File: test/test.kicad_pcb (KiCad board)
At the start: 2 copper layers, 100 x 100 mm, 107 parts, among them J1 UEXT_Host, J2 Conn_01x02, J3 Conn_02x06_Odd_Even, J4 Conn_02x06_Odd_Even, J5 Conn_02x06_Odd_Even, Q1 BC859, Q10 BC848, Q11 BC808, Q12 BC848, Q13 BC848, Q14 BC808, Q15 BC848, Q16 BC808, Q17 BC808, Q2 BC859, Q3 BC859, Q4 BC859, Q5 BC859, Q6 BC848, Q7 BC808, Q8 BC848, Q9 BC808, U3 PCA9531PW, U4 PCF8574AT, U6 TLC59108FPW

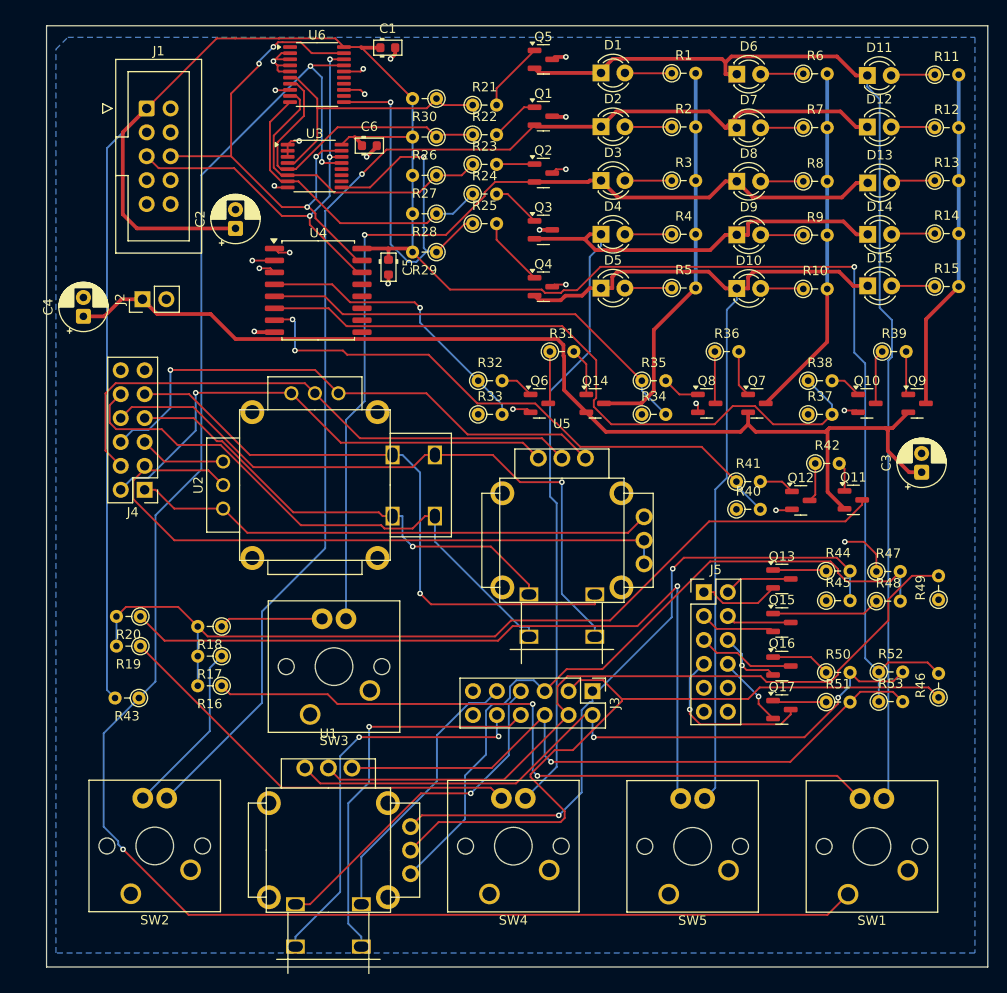
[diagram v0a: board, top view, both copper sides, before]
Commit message: work on 2nd update test
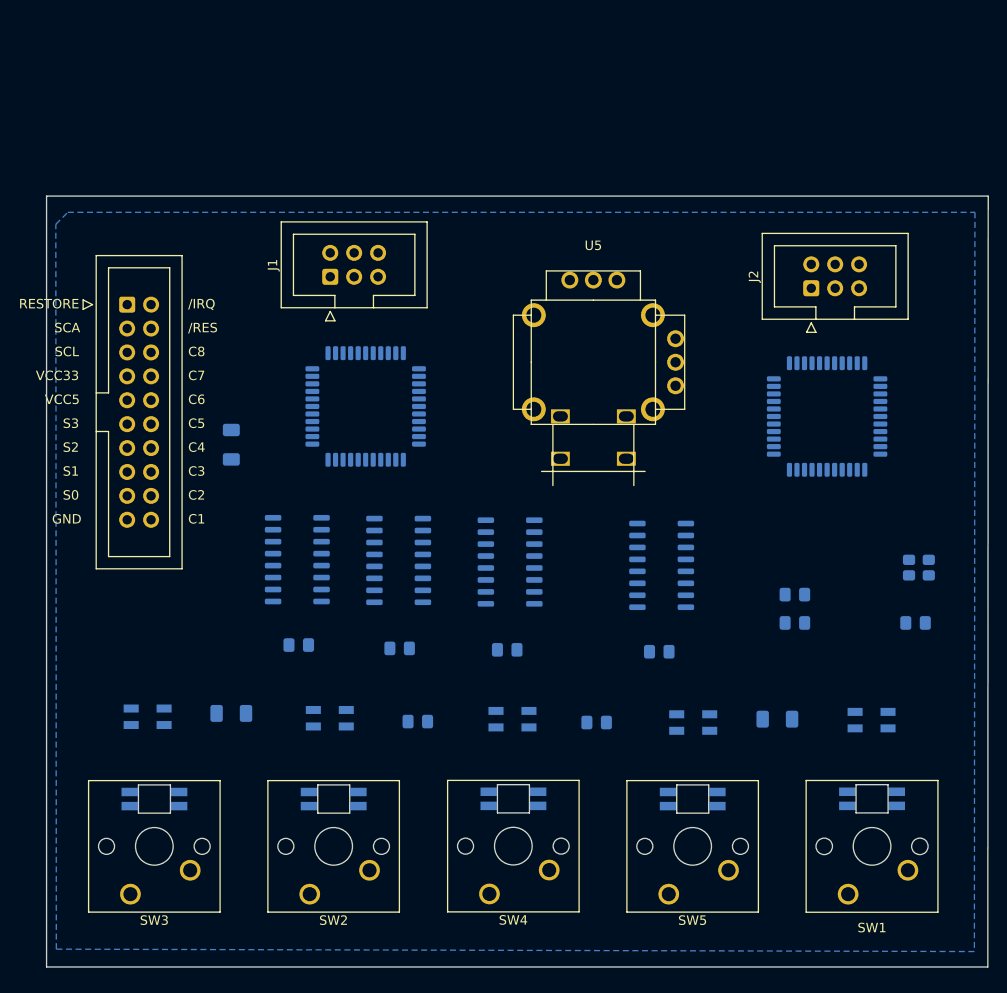
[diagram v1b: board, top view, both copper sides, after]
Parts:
- removed C1, C5, C6: C, PCM_Diode_SMD_Handsoldering_AKL:D_0603_1608Metric
- removed C2, C3, C4: C_Polarized, Capacitor_THT:CP_Radial_D5.0mm_P2.00mm
- removed D10, D11, D12, D13, D14, D15, D6, D7, D8, D9: LED, LED_THT:LED_D3.0mm
- removed J3, J4, J5: Conn_02x06_Odd_Even, Connector_PinHeader_2.54mm:PinHeader_2x06_P2.54mm_Vertical
- removed Q1, Q2, Q3, Q4, Q5: BC859, Package_TO_SOT_SMD:SOT-23
- removed Q10, Q12, Q13, Q15, Q6, Q8: BC848, Package_TO_SOT_SMD:SOT-23
- removed Q11, Q14, Q16, Q17, Q7, Q9: BC808, Package_TO_SOT_SMD:SOT-23
- removed R1, R10, R11, R12, R13, R14, R15, R16, R17, R18, R19, R2, R20, R3, R4, R5, R6, R7, R8, R9: R, Resistor_THT:R_Axial_DIN0204_L3.6mm_D1.6mm_P2.54mm_Vertical
- removed R21, R22, R23, R24, R25, R26, R27, R28, R29, R30, R31, R32, R33, R34, R35, R36, R37, R38, R39, R40, R41, R42, R43, R44, R45, R47, R48, R50, R51, R52, R53: 100k, Resistor_THT:R_Axial_DIN0204_L3.6mm_D1.6mm_P2.54mm_Vertical
- removed R46, R49: 1k, Resistor_THT:R_Axial_DIN0204_L3.6mm_D1.6mm_P2.54mm_Vertical
- removed U1: ~, petkn:THB Miniature Thumbstick THB001P
- added C10: 100n, Capacitor_SMD:C_0805_2012Metric_Pad1.18x1.45mm_HandSolder, B.Cu at (62.9, 127.3)
- added C11: 100n, Capacitor_SMD:C_0805_2012Metric_Pad1.18x1.45mm_HandSolder, B.Cu at (51.5, 127.2)
- added C12: 100n, Capacitor_SMD:C_0805_2012Metric_Pad1.18x1.45mm_HandSolder, B.Cu at (40.8, 126.8)
- added C13: 100n, Capacitor_SMD:C_0805_2012Metric_Pad1.18x1.45mm_HandSolder, B.Cu at (106.3, 124.4)
- added C14: 100n, Capacitor_SMD:C_0805_2012Metric_Pad1.18x1.45mm_HandSolder, B.Cu at (72.4, 135.0)
- added C15: 100u, Capacitor_SMD:C_1206_3216Metric_Pad1.33x1.80mm_HandSolder, B.Cu at (91.6, 134.7)
- added C16: 100u, Capacitor_SMD:C_1206_3216Metric_Pad1.33x1.80mm_HandSolder, B.Cu at (33.6, 134.1)
- added C17: 100n, Capacitor_SMD:C_0805_2012Metric_Pad1.18x1.45mm_HandSolder, B.Cu at (53.4, 134.9)
- added C18: 100u, Capacitor_SMD:C_1206_3216Metric_Pad1.33x1.80mm_HandSolder, B.Cu at (33.6, 105.5)
- added C7: 100n, Capacitor_SMD:C_0805_2012Metric_Pad1.18x1.45mm_HandSolder, B.Cu at (93.5, 124.4)
- added C8: 100n, Capacitor_SMD:C_0805_2012Metric_Pad1.18x1.45mm_HandSolder, B.Cu at (93.5, 121.4)
- added C9: 100n, Capacitor_SMD:C_0805_2012Metric_Pad1.18x1.45mm_HandSolder, B.Cu at (79.1, 127.5)
- added J6: New_PET_keyboard_connector, petkn:PET_New_Keyboard_Connector, F.Cu at (25.1, 100.8)
- added U7: 74LS145, Package_SO:SO-16_3.9x9.9mm_P1.27mm, B.Cu at (79.3, 118.3)
- added U8: ATmega32A-A, Package_QFP:TQFP-44_10x10mm_P0.8mm, B.Cu at (96.9, 102.5)
- added Y1: ASE-xxxMHz, Oscillator:Oscillator_SMD_Abracon_ASE-4Pin_3.2x2.5mm, B.Cu at (106.7, 118.6)
- D1, D2, D3, D4, D5: value LED -> SK6812MINI; footprint LED_THT:LED_D3.0mm -> LED_SMD:LED_SK6812MINI_PLCC4_3.5x3.5mm_P1.75mm; moved to B.Cu
- J1: value UEXT_Host -> AVR-ISP-6; footprint Connector_IDC:IDC-Header_2x05_P2.54mm_Vertical -> Connector_IDC:IDC-Header_2x03_P2.54mm_Vertical
- J2: value Conn_01x02 -> AVR-ISP-6; footprint Connector_PinHeader_2.54mm:PinHeader_1x02_P2.54mm_Vertical -> Connector_IDC:IDC-Header_2x03_P2.54mm_Vertical
- SW1: footprint petkn:SW_Cherry_MX_1.00u_PCB_with_LED -> CherryMX_PCB_LTST-A683CEGBW-Rotated:CherryMX_1.00u_PCB_LTST-A683CEGBW-Rotated
- SW2: value ~ -> CherryMX_LTST-A683CEGBW; footprint petkn:SW_Cherry_MX_1.00u_PCB_with_LED -> petkn:SW_Cherry_MX_1.00u_PCB_with_RGB_LED
- SW3, SW4, SW5: footprint petkn:SW_Cherry_MX_1.00u_PCB_with_LED -> petkn:SW_Cherry_MX_1.00u_PCB_with_RGB_LED
- U2: value ~ -> ATmega32A-A; footprint petkn:true-components-98002c3-ps2-ps3 -> Package_QFP:TQFP-44_10x10mm_P0.8mm; moved to B.Cu
- U3: value PCA9531PW -> 74HCT85; footprint Package_SO:TSSOP-16_4.4x5mm_P0.65mm -> Package_SO:SO-16_3.9x9.9mm_P1.27mm; moved to B.Cu
- U4: value PCF8574AT -> 74LS174; footprint Package_SO:SOIC-16W_7.5x10.3mm_P1.27mm -> Package_SO:SO-16_3.9x9.9mm_P1.27mm; moved to B.Cu
- U6: value TLC59108FPW -> 74LS174; footprint Package_SO:TSSOP-20_4.4x6.5mm_P0.65mm -> Package_SO:SO-16_3.9x9.9mm_P1.27mm; moved to B.Cu
- moved D2 79.1 mm to (24.7, 134.4)
- moved D1 74.4 mm to (44.1, 134.6)
- moved J2 71.1 mm to (95.2, 88.9)
- moved D3 58.0 mm to (63.5, 134.7)
- moved D5 54.2 mm to (101.7, 134.8)
- moved D4 52.8 mm to (82.7, 135.0)
- moved U6 51.6 mm to (40.6, 117.7)
- moved U3 46.9 mm to (63.2, 118.0)
- moved U4 29.9 mm to (51.4, 117.8)
- moved SW3 27.0 mm to (22.9, 153.3)
- moved J1 26.5 mm to (44.1, 87.7), turned to 90 degrees
- moved U5 19.2 mm to (72.1, 96.8)
- moved SW2 19.0 mm to (42.0, 153.3)
- moved U2 9.94 mm to (47.9, 101.4), turned to -90 degrees
- moved SW1 5.69 mm to (101.7, 148.2)
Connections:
- D1 pad 1: Net-(D1-K) -> Net-(D1-DOUT)
- D1 pad 2: Net-(D1-A) -> GND
- D2 pad 1: Net-(D12-K) -> Net-(D1-DIN)
- D2 pad 2: Net-(D2-A) -> GND
- D3 pad 1: Net-(D13-K) -> Net-(D3-DOUT)
- D3 pad 2: Net-(D3-A) -> GND
- D4 pad 1: Net-(D14-K) -> Net-(D4-DOUT)
- D4 pad 2: Net-(D4-A) -> GND
- D5 pad 1: Net-(D10-K) -> unconnected-(D5-DOUT-Pad1)
- D5 pad 2: Net-(D5-A) -> GND
- J1 pad 1: VCC -> Net-(J1-MISO)
- J1 pad 2: GND -> VCC
- J1 pad 3: unconnected-(J1-TXD-Pad3) -> Net-(J1-SCK)
- J1 pad 4: unconnected-(J1-RXD-Pad4) -> Net-(J1-MOSI)
- J1 pad 5: SCL -> Net-(J1-~{RST})
- J1 pad 6: SDA -> GND
- J2 pad 1: VCC5 -> Net-(J2-MISO)
- J2 pad 2: GND -> VCC
- SW1 pad 1: /RES -> Col1
- SW1 pad 2: GND -> Row0
- SW1 pad 3: Net-(D1-K) -> GND
- SW1 pad 4: Net-(R16-Pad1) -> Net-(SW1B-DIN)
- SW2 pad 3: Net-(D12-K) -> GND
- SW2 pad 4: Net-(R17-Pad1) -> Net-(SW1B-DOUT)
- SW3 pad 1: unconnected-(SW3-Pad1) -> Col5
- SW3 pad 2: unconnected-(SW3-Pad2) -> Row0
- SW3 pad 3: Net-(D13-K) -> GND
- SW4 pad 1: unconnected-(SW4-Pad1) -> Col5
- SW4 pad 2: unconnected-(SW4-Pad2) -> Row8
- SW4 pad 3: Net-(D14-K) -> GND
- SW4 pad 4: Net-(R19-Pad1) -> Net-(SW3B-DOUT)
- SW5 pad 1: unconnected-(SW5-Pad1) -> Col1
- SW5 pad 2: unconnected-(SW5-Pad2) -> Row8
- SW5 pad 3: Net-(D10-K) -> GND
- SW5 pad 4: Net-(R20-Pad1) -> Net-(SW4B-DOUT)
- U2 pad 1: (no net) -> Net-(J1-MOSI)
- U2 pad 10: Net-(J4-Pin_3) -> Net-(U2-PD1)
- U2 pad 11: Net-(J4-Pin_5) -> Net-(U2-PD2)
- U2 pad 12: Net-(J4-Pin_2) -> Net-(U2-PB4)
- U2 pad 13: Net-(J4-Pin_4) -> Col4
- U2 pad 14: Net-(J4-Pin_6) -> Col5
- U2 pad 2: (no net) -> Net-(J1-MISO)
- U2 pad 3: (no net) -> Net-(J1-SCK)
- U2 pad 4: (no net) -> Net-(J1-~{RST})
- U2 pad 5: Net-(J4-Pin_9) -> VCC
- U2 pad 6: Net-(J4-Pin_7) -> GND
- U2 pad 7: Net-(J4-Pin_10) -> unconnected-(U2-XTAL2-Pad7)
- U2 pad 8: Net-(J4-Pin_8) -> CLK16M
- U2 pad 9: Net-(J4-Pin_1) -> Net-(U2-PD0)
- U3 pad 1: GND -> S3
- U3 pad 10: unconnected-(U3-LED5-Pad10) -> Net-(U3-A0)
- U3 pad 11: unconnected-(U3-LED6-Pad11) -> S1
- U3 pad 12: unconnected-(U3-LED7-Pad12) -> Net-(U3-A1)
- U3 pad 13: /RES -> Net-(U3-A2)
- U3 pad 14: SCL -> S2
- U3 pad 15: SDA -> Net-(U3-A3)
- U3 pad 2: GND -> unconnected-(U3-Ia<b-Pad2)
- U3 pad 3: GND -> VCC
- U3 pad 4: PWM0 -> unconnected-(U3-Ia>b-Pad4)
- U3 pad 5: PWM1 -> unconnected-(U3-Oa>b-Pad5)
- U3 pad 6: PWM2 -> Net-(U2-PD2)
- U3 pad 7: PWM3 -> unconnected-(U3-Oa<b-Pad7)
- U3 pad 9: PWM4 -> S0
- U4 pad 1: GND -> VCC
- U4 pad 10: unconnected-(U4-P5-Pad10) -> Net-(U3-A2)
- U4 pad 11: unconnected-(U4-P6-Pad11) -> Net-(U4-D3)
- U4 pad 12: unconnected-(U4-P7-Pad12) -> Net-(U3-A1)
- U4 pad 13: unconnected-(U4-~{INT}-Pad13) -> Net-(U4-D4)
- U4 pad 14: SCL -> Net-(U4-D5)
- U4 pad 15: SDA -> Net-(U3-A0)
- U4 pad 2: GND -> Net-(U4-D3)
- U4 pad 3: GND -> Net-(U4-D0)
- U4 pad 4: ON0 -> Net-(U4-D1)
- U4 pad 5: ON1 -> Net-(U4-D2)
- U4 pad 6: ON2 -> Net-(U4-D2)
- U4 pad 7: ON3 -> Net-(U3-A3)
- U4 pad 9: unconnected-(U4-P4-Pad9) -> CLK16M
- U5 pad 10: Net-(J4-Pin_4) -> Col2
- U5 pad 11: Net-(J4-Pin_6) -> Row5
- U5 pad 12: Net-(J4-Pin_1) -> Row3
- U5 pad 13: Net-(J4-Pin_3) -> Col2
- U5 pad 14: Net-(J4-Pin_3) -> Row4
- U5 pad 5: Net-(J4-Pin_9) -> unconnected-(U5C-SW1_A-Pad5)
- U5 pad 6: Net-(J4-Pin_7) -> unconnected-(U5C-SW1_B-Pad6)
- U5 pad 7: Net-(J4-Pin_10) -> Col4
- U5 pad 8: Net-(J4-Pin_8) -> Row1
- U5 pad 9: Net-(J4-Pin_2) -> Row7
- U6 pad 1: unconnected-(U6-REXT-Pad1) -> VCC
- U6 pad 10: PWM3 -> Net-(U4-D1)
- U6 pad 11: PWM4 -> S3
- U6 pad 12: IO5 -> Net-(U4-D4)
- U6 pad 13: GND -> Net-(U6-D4)
- U6 pad 14: IO6 -> Net-(U6-D5)
- U6 pad 15: IO7 -> Net-(U4-D5)
- U6 pad 16: GND -> VCC
- U6 pad 2: GND -> Net-(U6-D5)
- U6 pad 3: GND -> S0
- U6 pad 4: GND -> S1
- U6 pad 5: GND -> Net-(U6-D4)
- U6 pad 6: PWM0 -> S2
- U6 pad 7: PWM1 -> Net-(U4-D0)
- U6 pad 9: PWM2 -> CLK16M
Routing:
- net VCC: track 262.3 -> 0.00 mm, vias 1 -> 0
- net /RES: track 190.4 -> 0.00 mm, vias 3 -> 0
- net Net-(D12-K): track 134.9 -> 0.00 mm, vias 1 -> 0
- net Net-(D1-K): track 118.3 -> 0.00 mm
- net VCC5: track 116.2 -> 0.00 mm
- net Net-(D14-K): track 104.2 -> 0.00 mm
- net Net-(D13-K): track 100.8 -> 0.00 mm, vias 1 -> 0
- net Net-(Q11-C): track 96.7 -> 0.00 mm
- net Net-(D10-K): track 96.2 -> 0.00 mm
- net Net-(R20-Pad1): track 83.2 -> 0.00 mm, vias 1 -> 0
- net Net-(J3-Pin_4): track 79.8 -> 0.00 mm
- net Net-(J3-Pin_3): track 78.6 -> 0.00 mm
- net Net-(J3-Pin_5): track 77.6 -> 0.00 mm
- net Net-(R16-Pad1): track 77.0 -> 0.00 mm, vias 2 -> 0
- net Net-(J3-Pin_2): track 74.4 -> 0.00 mm, vias 2 -> 0
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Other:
- board size 100 x 100 mm -> 100 x 81.9 mm
